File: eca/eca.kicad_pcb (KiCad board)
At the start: 2 copper layers, 60 x 61.5 mm, 22 parts, among them J1 RPI Bus, J10 ESP32CAM Power Supply Bus, J11 28BYJ48 1 Power Supply Bus, J12 28BYJ48 2 Power Supply Bus, J13 28BYJ48 3 Power Supply Bus, J15 Fan 1 Power Supply Bus, J16 Fan Power Supply Bus, J2 GY 906 Bus, J3 MAX30102 Bus, J4 TCRT5000 1 Bus, J5 TCRT5000 2 Bus, J7 28BYJ48 1 Control Bus, J8 28BYJ48 2 Control Bus, J9 28BYJ48 3 Control Bus

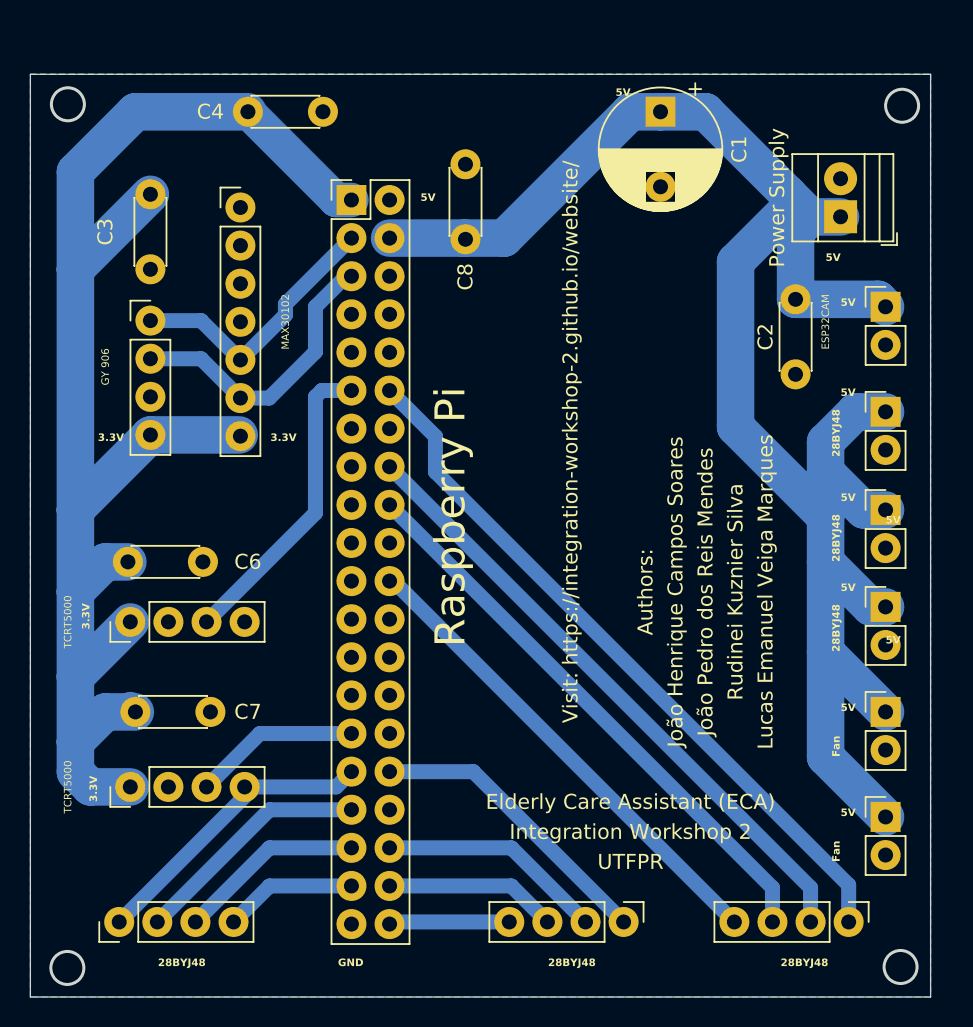
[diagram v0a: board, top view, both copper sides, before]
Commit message: alpha version
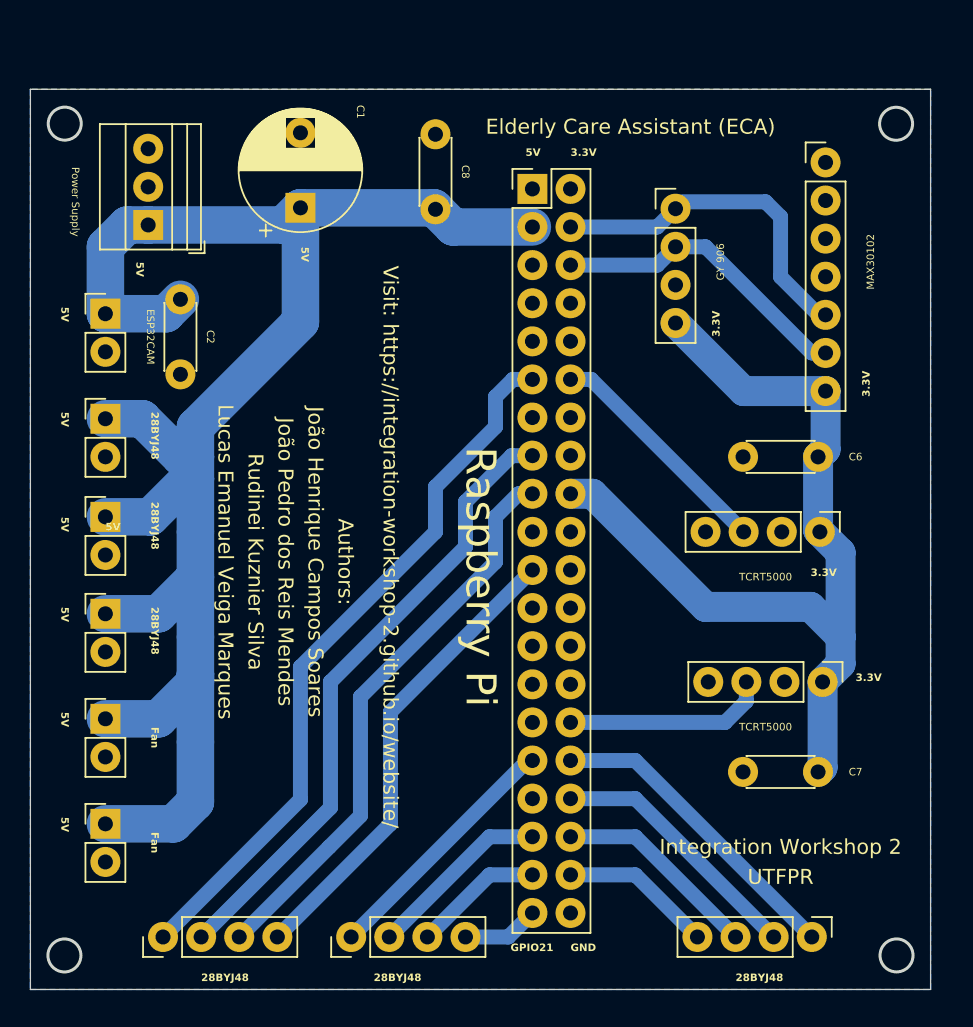
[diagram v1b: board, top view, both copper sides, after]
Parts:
- removed C3, C4: 100nF, Capacitor_THT:C_Disc_D4.3mm_W1.9mm_P5.00mm
- removed Power Supply: Power Supply Input, TerminalBlock:TerminalBlock_Xinya_XY308-2.54-2P_1x02_P2.54mm_Horizontal
- added J6: Power Supply Input, TerminalBlock:TerminalBlock_Xinya_XY308-2.54-3P_1x03_P2.54mm_Horizontal, F.Cu at (107.8, 81.5)
- moved J10 52.0 mm to (105.0, 87.5)
- moved J11 52.0 mm to (105.0, 107.5)
- moved J12 52.0 mm to (105.0, 101.0)
- moved J13 52.0 mm to (105.0, 94.5)
- moved J15 52.0 mm to (105.0, 121.5)
- moved J16 52.0 mm to (105.0, 114.5)
- moved J4 46.7 mm to (152.8, 112.0), turned to -90 degrees
- moved C6 46.5 mm to (152.5, 97.0), turned to 180 degrees
- moved J5 46.3 mm to (152.6, 102.0), turned to -90 degrees
- moved J7 46.2 mm to (152.1, 129.0), turned to -90 degrees
- moved J8 45.7 mm to (108.8, 129.0), turned to 90 degrees
- moved C7 45.7 mm to (152.5, 118.0), turned to 180 degrees
- moved C2 41.0 mm to (110.0, 86.5)
- moved J3 39.1 mm to (153.0, 77.4)
- moved J2 35.8 mm to (143.0, 80.5)
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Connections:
- J1 pad 1: 3.3V -> 5V
- J1 pad 10: GPIO15 -> GND
- J1 pad 11: GPIO17 -> GPIO18
- J1 pad 12: GPIO18 -> GPIO17
- J1 pad 13: GPIO27 -> GND
- J1 pad 14: GND -> GPIO27
- J1 pad 15: GPIO22 -> GPIO23
- J1 pad 16: GPIO23 -> GPIO22
- J1 pad 17: 3.3V -> GPIO24
- J1 pad 18: GPIO24 -> 3.3V
- J1 pad 19: GPIO10 -> GND
- J1 pad 2: 5V -> 3.3V
- J1 pad 20: GND -> GPIO10
- J1 pad 21: GPIO9 -> GPIO25
- J1 pad 22: GPIO25 -> GPIO9
- J1 pad 23: GPIO11 -> GPIO8
- J1 pad 24: GPIO8 -> GPIO11
- J1 pad 25: GND -> GPIO7
- J1 pad 26: GPIO7 -> GND
- J1 pad 27: ID_SD -> ID_SC
- J1 pad 28: ID_SC -> ID_SD
- J1 pad 29: GPIO5 -> GND
- J1 pad 3: GPIO2 -> 5V
- J1 pad 30: GND -> GPIO5
- J1 pad 31: GPIO6 -> GPIO12
- J1 pad 32: GPIO12 -> GPIO6
- J1 pad 33: GPIO13 -> GND
- J1 pad 34: GND -> GPIO13
- J1 pad 35: GPIO19 -> GPIO16
- J1 pad 36: GPIO16 -> GPIO19
- J1 pad 37: GPIO26 -> GPIO20
- J1 pad 38: GPIO20 -> GPIO26
- J1 pad 39: GND -> GPIO21
- J1 pad 4: 5V -> GPIO2
- J1 pad 40: GPIO21 -> GND
- J1 pad 5: GPIO3 -> GND
- J1 pad 6: GND -> GPIO3
- J1 pad 7: GPIO4 -> GPIO14
- J1 pad 8: GPIO14 -> GPIO4
- J1 pad 9: GND -> GPIO15
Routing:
- net 3.3V: track 102.6 -> 60.8 mm
- net GPIO2: track 18.3 -> 23.2 mm
- net GPIO17: track 20.6 -> 15.7 mm
- net 5V: track 122.5 -> 118.5 mm
- net GPIO21: track 8.04 -> 5.12 mm
- net GPIO20: track 11.5 -> 8.71 mm
- net GPIO16: track 15.1 -> 12.3 mm
- net GPIO12: track 19.8 -> 17.0 mm
- net GPIO5: track 11.3 -> 13.6 mm
- net GPIO3: track 19.6 -> 21.1 mm
- net GPIO6: track 19.6 -> 21.0 mm
- net GPIO26: track 8.85 -> 10.2 mm
- net GPIO19: track 12.4 -> 13.8 mm
- net GPIO13: track 16.0 -> 17.4 mm
- net GPIO25: track 32.4 -> 31.5 mm
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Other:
- board size 60 x 61.5 mm -> 60 x 60 mm
- board text added: "C1"
- board text added: "C2"
- board text added: "C6"
- board text added: "C7"
- board text added: "C8"
- board text added: "GPIO21"
- board text added: "Power Supply"
